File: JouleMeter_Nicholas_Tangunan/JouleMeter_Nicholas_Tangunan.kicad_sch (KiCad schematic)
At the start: 33 parts, among them J1 22035035, J2 22035035, SW1 SW_SPDT, SW2 SW_SPDT

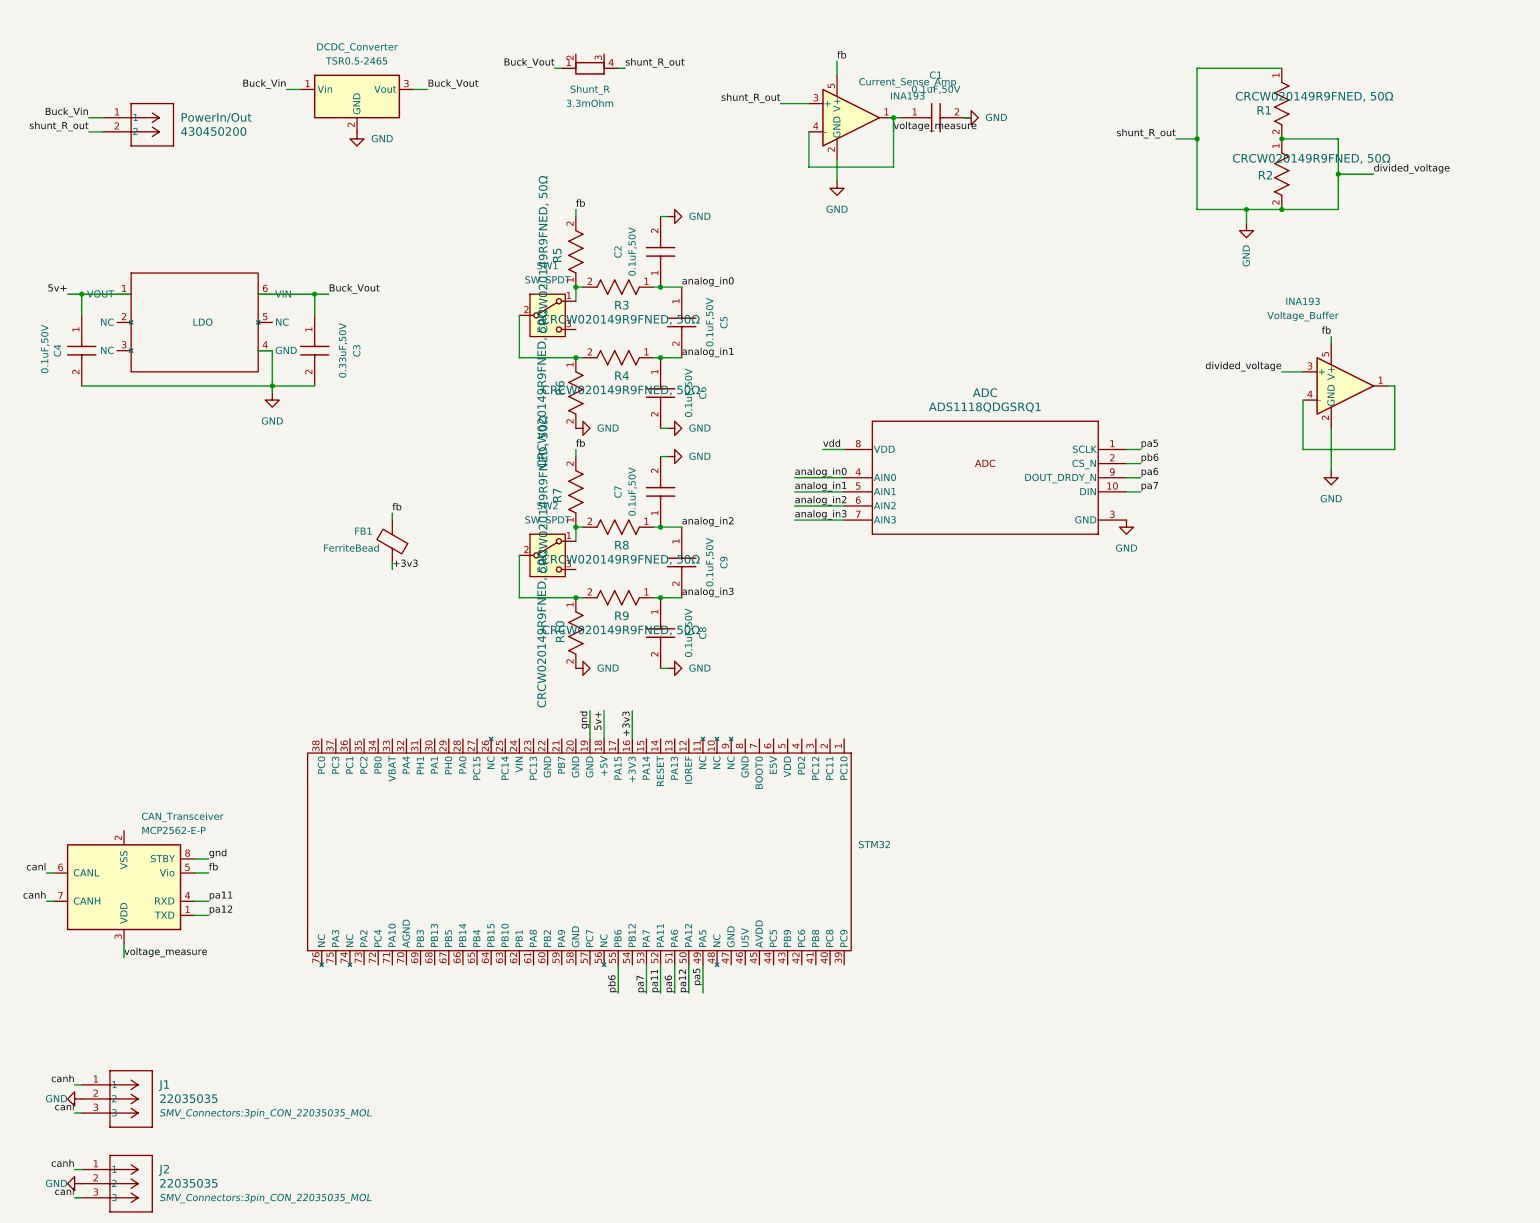
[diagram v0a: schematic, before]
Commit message: updated schematic
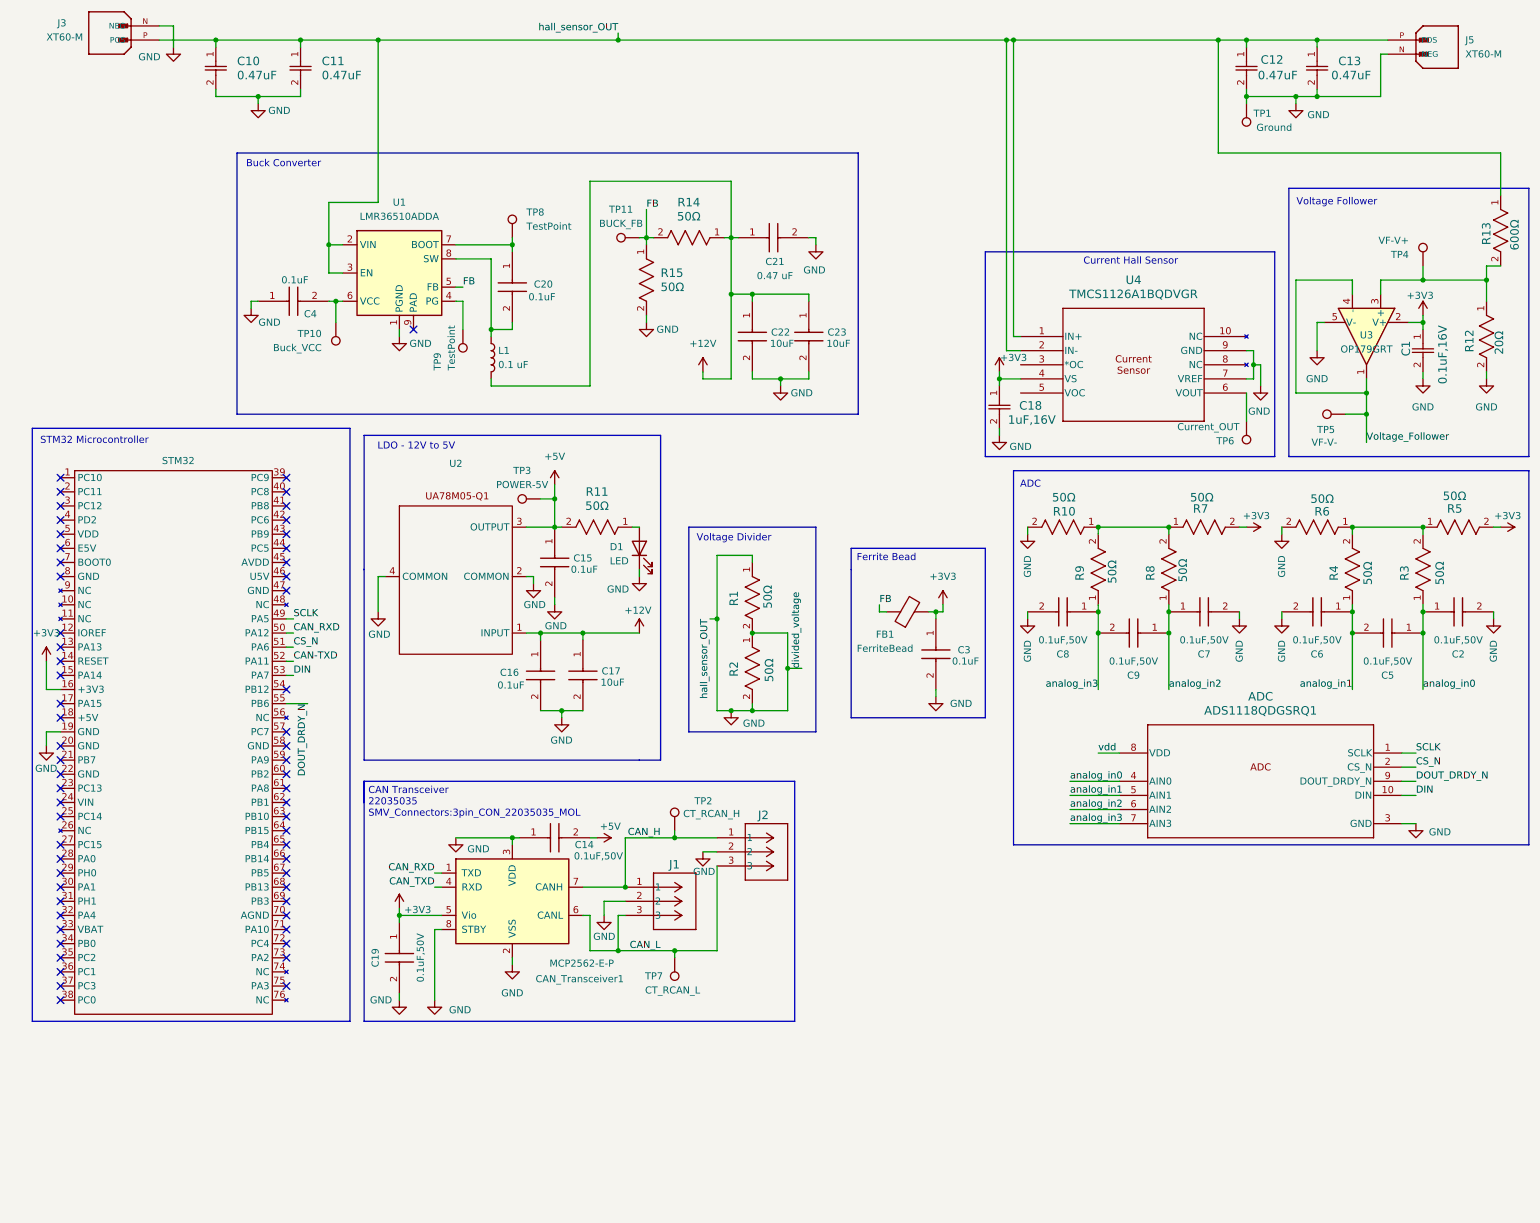
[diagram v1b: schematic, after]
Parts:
- removed C1: 0.1uF,50V, SMV_Passives:Cap0805, symbol SMV_Custom:C0805C104K5RACTU
- removed C3: 0.33uF,50V, SMV_Passives:Cap0805, symbol SMV_Custom:C0805C334K5RACTU
- removed CAN_Transceiver: MCP2562-E-P, Package_DIP:DIP-8_W7.62mm, symbol Interface_CAN_LIN:MCP2562-E-P
- removed Current_Sense_Amp, Voltage_Buffer: INA193, Package_TO_SOT_SMD:SOT-23-5, symbol Amplifier_Current:INA193
- removed DCDC_Converter: TSR0.5-2465, Converter_DCDC:Converter_DCDC_TRACO_TSR0.5-24xx_TSR0.5-24xxx_THT, symbol Regulator_Switching:TSR0.5-2465
- removed LDO: ~, symbol SMV_Custom:AP7387-50FDCR-7
- removed PowerIn/Out: 430450200, SMV_Connectors:CONN_SD-43045-001_02_MOL, symbol SMV_Custom:430450200
- removed SW1, SW2: SW_SPDT, symbol Switch:SW_SPDT
- removed Shunt_R: 3.3mOhm, symbol Device:R_Shunt
- added C1: 0.1uF,16V, SMV_Passives:Cap0805, symbol SMV_Custom:C0805C105K4RACTU
- added C10, C11, C12, C13: 0.47uF, SMV_Passives:CAPC340270_105N_KEM, symbol SMV_Custom:C1210C474K5RACTU
- added C14, C19: 0.1uF,50V, SMV_Passives:Cap0805, symbol SMV_Custom:C0805C104K5RACTU
- added C15, C16, C20, C3: 0.1uF, SMV_Passives:Cap0805, symbol SMV_Custom:C0805C104K5RACTU
- added C17, C22, C23: 10uF, SMV_Passives:Cap0805, symbol SMV_Custom:C0805C104K5RACTU
- added C18: 1uF,16V, SMV_Passives:Cap0805, symbol SMV_Custom:C0805C105K4RACTU
- added C21: 0.47 uF, SMV_Passives:Cap0805, symbol SMV_Custom:C0805C104K5RACTU
- added CAN_Transceiver1: MCP2562-E-P, Package_DIP:DIP-8_W7.62mm, symbol Interface_CAN_LIN:MCP2562-E-P
- added D1: LED, symbol Device:LED
- added J3, J5: XT60-M, SMV_Connectors:AMASS_XT60-M, symbol SMV_Custom:XT60-M
- added L1: 0.1 uF, symbol Device:L
- added R11, R14, R15: 50Ω, SMV_Passives:0805RESC2012X60N, symbol SMV_Custom:CRCW020149R9FNED
- added R12: 20Ω, SMV_Passives:0805RESC2012X60N, symbol SMV_Custom:CRCW020149R9FNED
- added R13: 600Ω, SMV_Passives:0805RESC2012X60N, symbol SMV_Custom:CRCW020149R9FNED
- added TP1: Ground, symbol Connector:TestPoint
- added TP10: Buck_VCC, symbol Connector:TestPoint
- added TP11: BUCK_FB, symbol Connector:TestPoint
- added TP2: CT_RCAN_H, symbol Connector:TestPoint
- added TP3: POWER-5V, symbol Connector:TestPoint
- added TP4: VF-V+, symbol Connector:TestPoint
- added TP5: VF-V-, symbol Connector:TestPoint
- added TP6: Current_OUT, symbol Connector:TestPoint
- added TP7: CT_RCAN_L, symbol Connector:TestPoint
- added TP8, TP9: TestPoint, symbol Connector:TestPoint
- added U1: LMR36510ADDA, Package_SO:Texas_HTSOP-8-1EP_3.9x4.9mm_P1.27mm_EP2.95x4.9mm_Mask2.4x3.1mm_ThermalVias, symbol Regulator_Switching:LMR36510ADDA
- added U2: ~, symbol SMV_Custom:UA78M05-Q1
- added U3: OP179GRT, Package_TO_SOT_SMD:SOT-23-5, symbol Amplifier_Operational:OP179GRT
- added U4: TMCS1126A1BQDVGR, SOIC10_DVG_TEX, symbol SMV_Custom:PMCS1126A1BQDVGR
- C4: value 0.1uF,50V -> 0.1uF
- J1: footprint SMV_Connectors:3pin_CON_22035035_MOL -> (none)
- R1, R10, R2, R3, R4, R5, R6, R7, R8, R9: value CRCW020149R9FNED, 50Ω -> 50Ω
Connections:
- net fb is gone; now on net +3V3: FB1.2, R5.2, R7.2
- net gnd is gone; now on net GND: STM32.19 (GND)
- net GND: now also C4.1, C1.2, C10.1, C10.2, C11.1, C11.2, C12.1, C12.2, C13.1, C13.2, C14.1, C15.2, C16.2, C17.2, C18.2, C19.2, C21.2, C22.2, C23.2, C3.2, CAN_Transceiver1.2 (VSS), CAN_Transceiver1.3 (VDD), CAN_Transceiver1.8 (STBY), D1.1 (K), J3.N (NEG), J3.P (POS), J5.N (NEG), J5.P (POS), R12.2, R13.1, R15.2, TP1.1, U1.1 (PGND), U1.2 (VIN), U1.3 (EN), U2.2 (COMMON), U2.4 (COMMON), U3.5 (V-), U4.1 (IN+), U4.2 (IN-), U4.7 (VREF), U4.9 (GND); no longer C4.2
- net at R10.1, R9.2: now also R7.1, R8.2
- net at R4.2, R6.1: now also R3.2, R5.1
- net +3v3 renamed +3V3
- net +3V3: now also C1.1, C18.1, C19.1, C3.1, CAN_Transceiver1.5 (Vio), U3.2 (V+), U4.4 (VS); no longer FB1.1
- net 5v+: no longer names the net of STM32.18 (+5V)
- net 5v+: no longer C4.1
- net canh renamed CAN_H
- net CAN_H: now also CAN_Transceiver1.7 (CANH), TP2.1
- net canl renamed CAN_L
- net CAN_L: now also CAN_Transceiver1.6 (CANL), TP7.1
- net pa11 renamed CAN-TXD
- net pa12 renamed CAN_RXD
- net CAN_RXD: now also CAN_Transceiver1.1 (TXD)
- net pa5 renamed SCLK
- net pa6 renamed CS_N
- net CS_N: now also ADC.2 (CS_N); no longer ADC.9 (DOUT_DRDY_N)
- net pa7 renamed DIN
- net pb6 renamed DOUT_DRDY_N
- net DOUT_DRDY_N: now also ADC.9 (DOUT_DRDY_N); no longer ADC.2 (CS_N)
- new net: C4.2, TP10.1, U1.6 (VCC)
- new net: TP6.1, U4.6 (VOUT)
- new net: C20.2, L1.1, U1.8 (SW)
- new net: R12.1, R13.2, TP4.1, U3.3 (+)
- new net: TP9.1, U1.4 (PG)
- new net: C20.1, TP8.1, U1.7 (BOOT)
- new net: D1.2 (A), R11.1
- new net +12V: C16.1, C17.1, C21.1, C22.1, C23.1, L1.2, R14.1, U2.1 (INPUT)
- new net +5V: C14.2, C15.1, R11.2, TP3.1, U2.3 (OUTPUT)
- new net CAN_TXD: CAN_Transceiver1.4 (RXD)
- new net FB: FB1.1, R14.2, R15.1, TP11.1, U1.5 (FB)
- new net Voltage_Follower: TP5.1, U3.1, U3.4 (-)
- no-connect marks 0 -> 61
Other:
- note added: "ADC"
- note added: "Buck Converter"
- note added: "CAN Transceiver 22035035 SMV_Connectors:3pin_CON_22035035_MOL"
- note added: "Current Hall Sensor"
- note added: "Ferrite Bead"
- note added: "LDO - 12V to 5V"
- note added: "STM32 Microcontroller"
- note added: "Voltage Divider"
- note added: "Voltage Follower"
- moved on the sheet: ADC, C2, C5, C6, C7, C8, C9, J1, J2, R1, R10, R2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
